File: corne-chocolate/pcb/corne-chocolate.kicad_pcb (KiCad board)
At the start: 2 copper layers, 133.8 x 91.4 mm, 116 parts, among them J2 nice!view, J3 Battery, J4 Battery, SW1 1U, SW10 1U, SW11 1U, SW12 1U, SW13 1U, SW14 1U, SW15 1U, SW16 1U, SW17 1U, SW18 1U, SW19 1U, SW2 1U, SW20 1U, SW21 1.5U, SW22 SW_PUSH, SW23 SW_SPDT, SW3 1U, SW4 1U, SW5 1U, SW6 1U, SW7 1U, SW8 1U, SW9 1U, U1 ProMicro

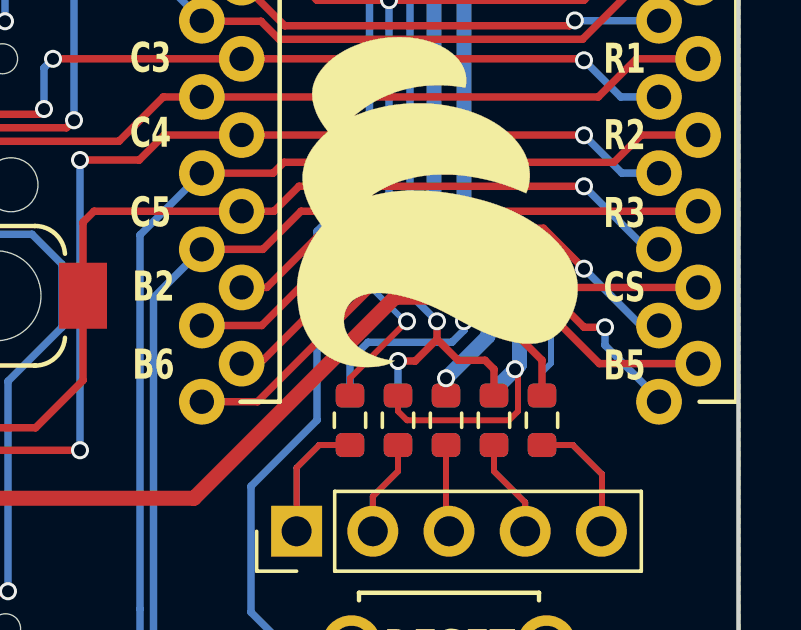
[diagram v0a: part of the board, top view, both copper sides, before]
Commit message: pcb clean up layout under MCU
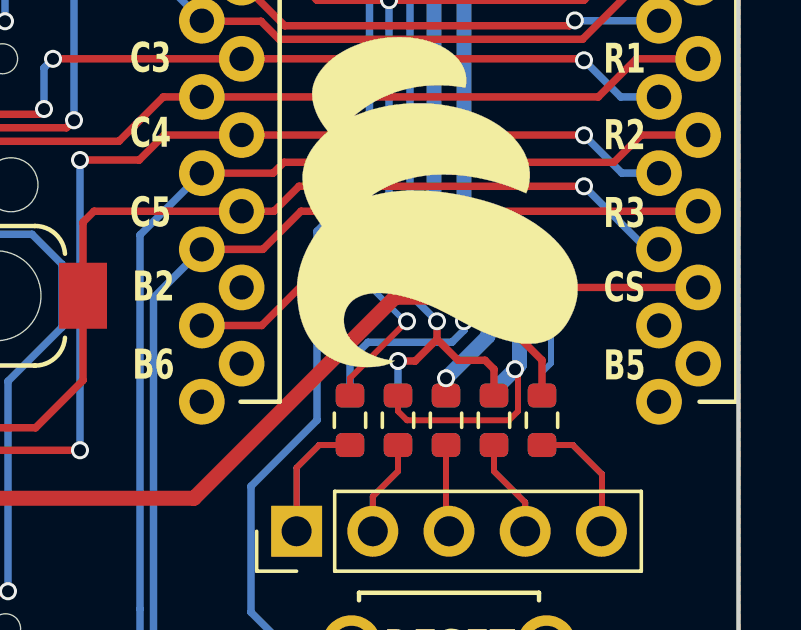
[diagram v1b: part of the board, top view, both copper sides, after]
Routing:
- net (no net): track 53.3 -> 0.00 mm, vias 2 -> 0
- net unconnected-(U1-16/PB2-Pad14): track 0.00 -> 0.61 mm
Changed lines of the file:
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@@
 	)
 	(segment
-		(start 187.3 96.2)
-		(end 182.3 96.2)
-		(width 0.25)
-		(layer "F.Cu")
-		(net 0)
-	)
-	(segment
-		(start 178.718 100.982)
-		(end 182.9 96.8)
-		(width 0.25)
-		(layer "F.Cu")
-		(net 0)
-	)
-	(segment
-		(start 188.2525 95.2)
-		(end 181 95.2)
-		(width 0.25)
-		(layer "F.Cu")
-		(net 0)
-	)
-	(segment
-		(start 190.112 99.712)
-		(end 193.4064 99.712)
-		(width 0.25)
-		(layer "F.Cu")
-		(net 0)
-	)
-	(segment
-		(start 182.3 96.2)
-		(end 178.788 99.712)
-		(width 0.25)
-		(layer "F.Cu")
-		(net 0)
-	)
-	(segment
-		(start 190.3 98.5)
-		(end 189.6 98.5)
-		(width 0.25)
-		(layer "F.Cu")
-		(net 0)
-	)
-	(segment
-		(start 187.2 96.8)
-		(end 190.112 99.712)
-		(width 0.25)
-		(layer "F.Cu")
-		(net 0)
-	)
-	(segment
-		(start 179.028 97.172)
-		(end 178.1864 97.172)
-		(width 0.25)
-		(layer "F.Cu")
-		(net 0)
-	)
-	(segment
-		(start 189.6 98.5)
-		(end 187.3 96.2)
-		(width 0.25)
-		(layer "F.Cu")
-		(net 0)
-	)
-	(segment
-		(start 178.788 99.712)
-		(end 178.1864 99.712)
-		(width 0.25)
-		(layer "F.Cu")
-		(net 0)
-	)
-	(segment
-		(start 176.86 100.982)
-		(end 178.718 100.982)
-		(width 0.25)
-		(layer "F.Cu")
-		(net 0)
-	)
-	(segment
-		(start 182.9 96.8)
-		(end 187.2 96.8)
-		(width 0.25)
-		(layer "F.Cu")
-		(net 0)
-	)
-	(segment
-		(start 181 95.2)
-		(end 179.028 97.172)
-		(width 0.25)
-		(layer "F.Cu")
-		(net 0)
-	)
-	(segment
-		(start 189.6 96.5475)
-		(end 188.2525 95.2)
-		(width 0.25)
-		(layer "F.Cu")
-		(net 0)
-	)
-	(via
-		(at 189.6 96.5475)
-		(size 0.6)
-		(drill 0.4)
-		(layers "F.Cu" "B.Cu")
-		(net 0)
-	)
-	(via
-		(at 190.3 98.5)
-		(size 0.6)
-		(drill 0.4)
-		(layers "F.Cu" "B.Cu")
-		(net 0)
-	)
-	(segment
-		(start 190.3 98.5)
-		(end 190.3 99.1)
-		(width 0.25)
-		(layer "B.Cu")
-		(net 0)
-	)
-	(segment
-		(start 192.1 100.9)
-		(end 192.1 100.982)
-		(width 0.25)
-		(layer "B.Cu")
-		(net 0)
-	)
-	(segment
-		(start 191.4945 98.442)
-		(end 192.1 98.442)
-		(width 0.25)
-		(layer "B.Cu")
-		(net 0)
-	)
-	(segment
-		(start 190.3 99.1)
-		(end 192.1 100.9)
-		(width 0.25)
-		(layer "B.Cu")
-		(net 0)
-	)
-	(segment
-		(start 189.6 96.5475)
-		(end 191.4945 98.442)
-		(width 0.25)
-		(layer "B.Cu")
-		(net 0)
-	)
-	(segment
 		(start 142.9 70.8)
 		(end 142.9 71.75)
@@
 		(net 75)
 	)
+	(segment
+		(start 192.1 100.9)
+		(end 192.1 100.982)
+		(width 0.25)
+		(layer "B.Cu")
+		(net 76)
+	)
+	(segment
+		(start 191.4945 98.442)
+		(end 192.1 98.442)
+		(width 0.25)
+		(layer "B.Cu")
+		(net 78)
+	)
 	(zone
